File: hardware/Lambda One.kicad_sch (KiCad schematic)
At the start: 8 parts, among them IC1 01, SW1 SW_Push, U1 W65C816SxP, U2 28C256, U3 ATF22V10C, U4 AS6C1008-xxP, U5 74HC74, Y1 TFT680

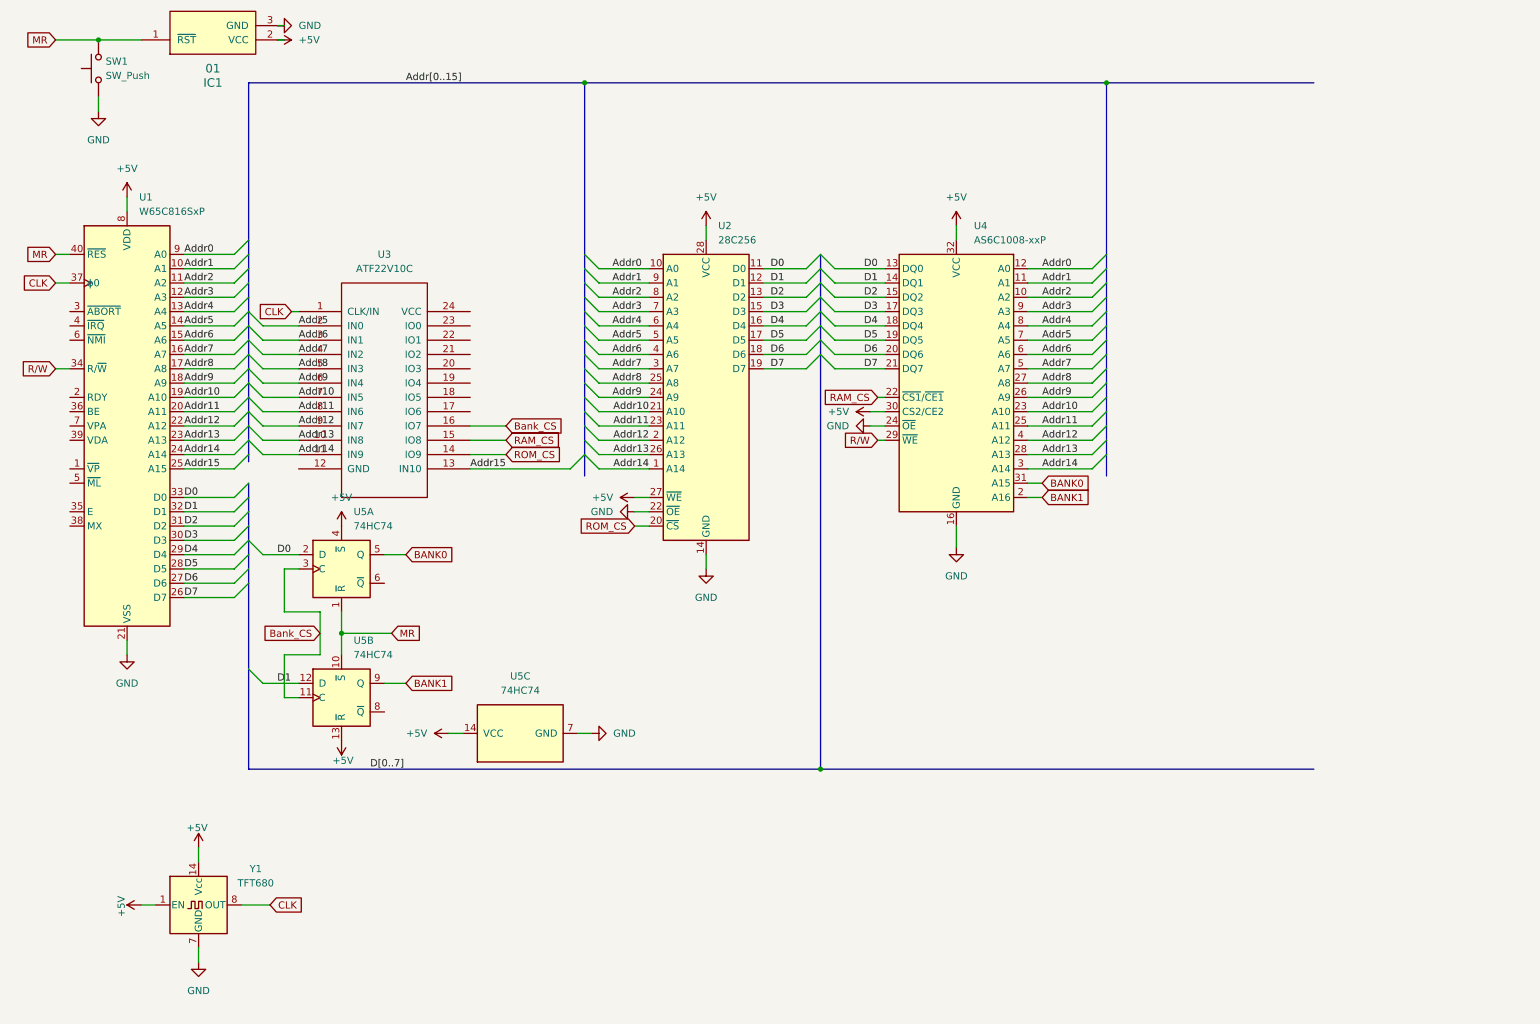
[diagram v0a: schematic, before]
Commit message: Modularized
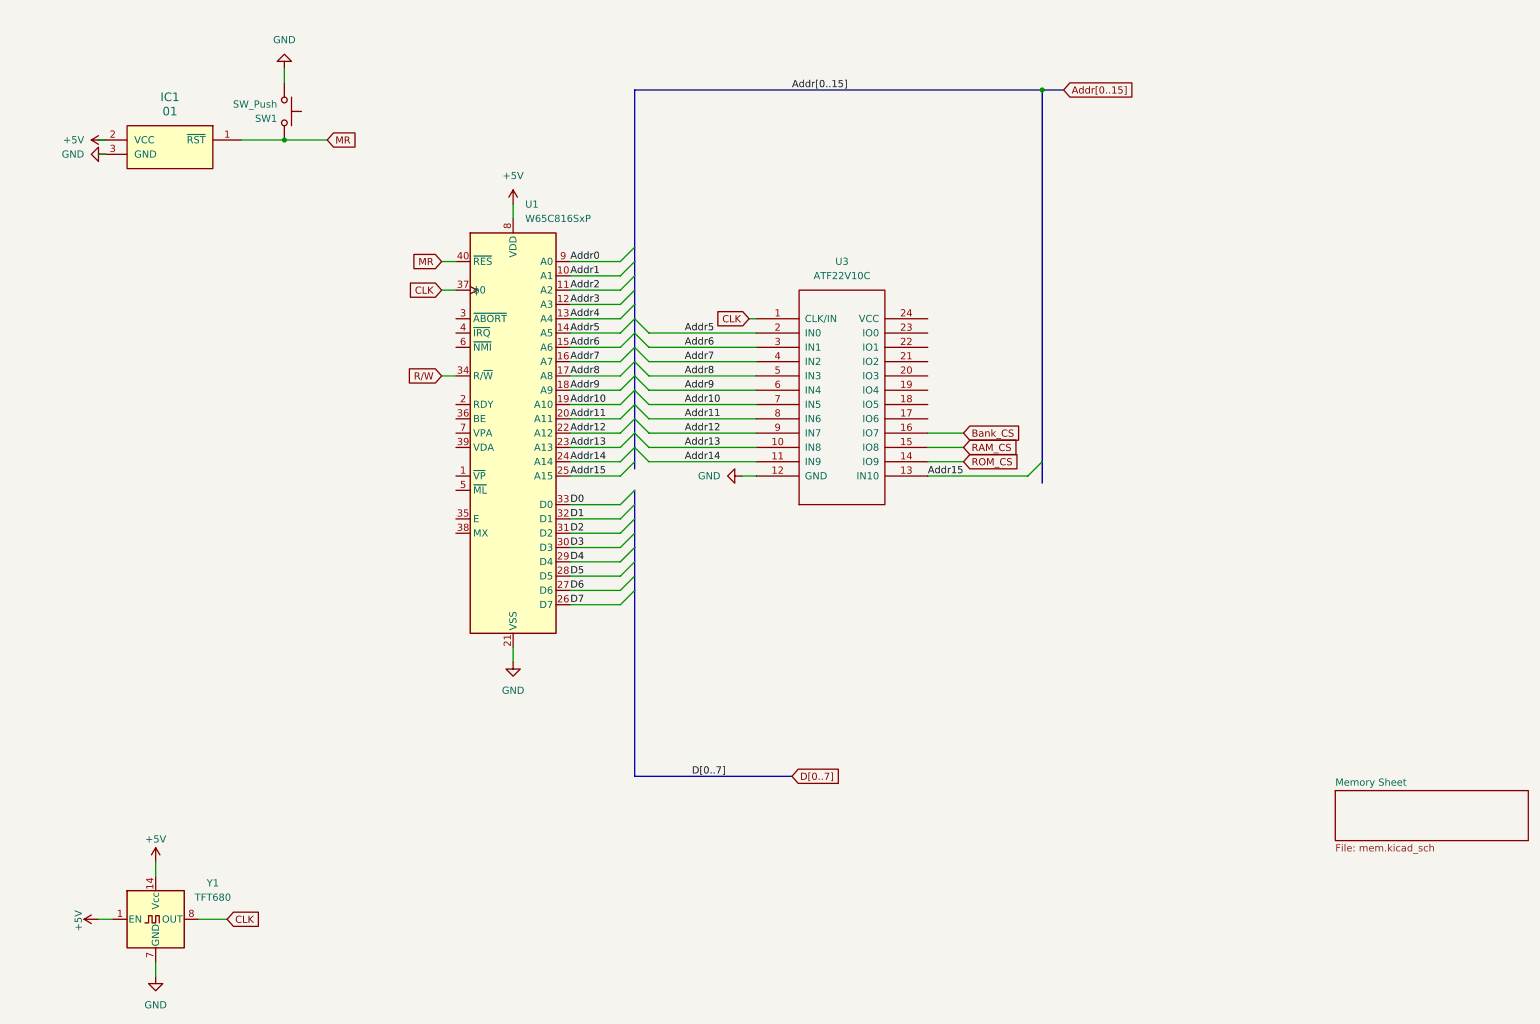
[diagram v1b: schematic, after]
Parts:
- removed U2: 28C256, symbol Memory_EEPROM:28C256
- removed U4: AS6C1008-xxP, Package_DIP:DIP-32_W15.24mm, symbol Memory_RAM:AS6C1008-xxP
- removed U5: 74HC74, symbol 74xx:74HC74
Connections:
- net GND: now also U3.12 (GND)
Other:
- added sheet Memory Sheet (mem.kicad_sch)
- moved on the sheet: IC1, SW1, U1, U3, Y1
